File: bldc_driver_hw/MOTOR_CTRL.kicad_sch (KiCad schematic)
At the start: 18 parts, among them U3 DRV8328BRUYR

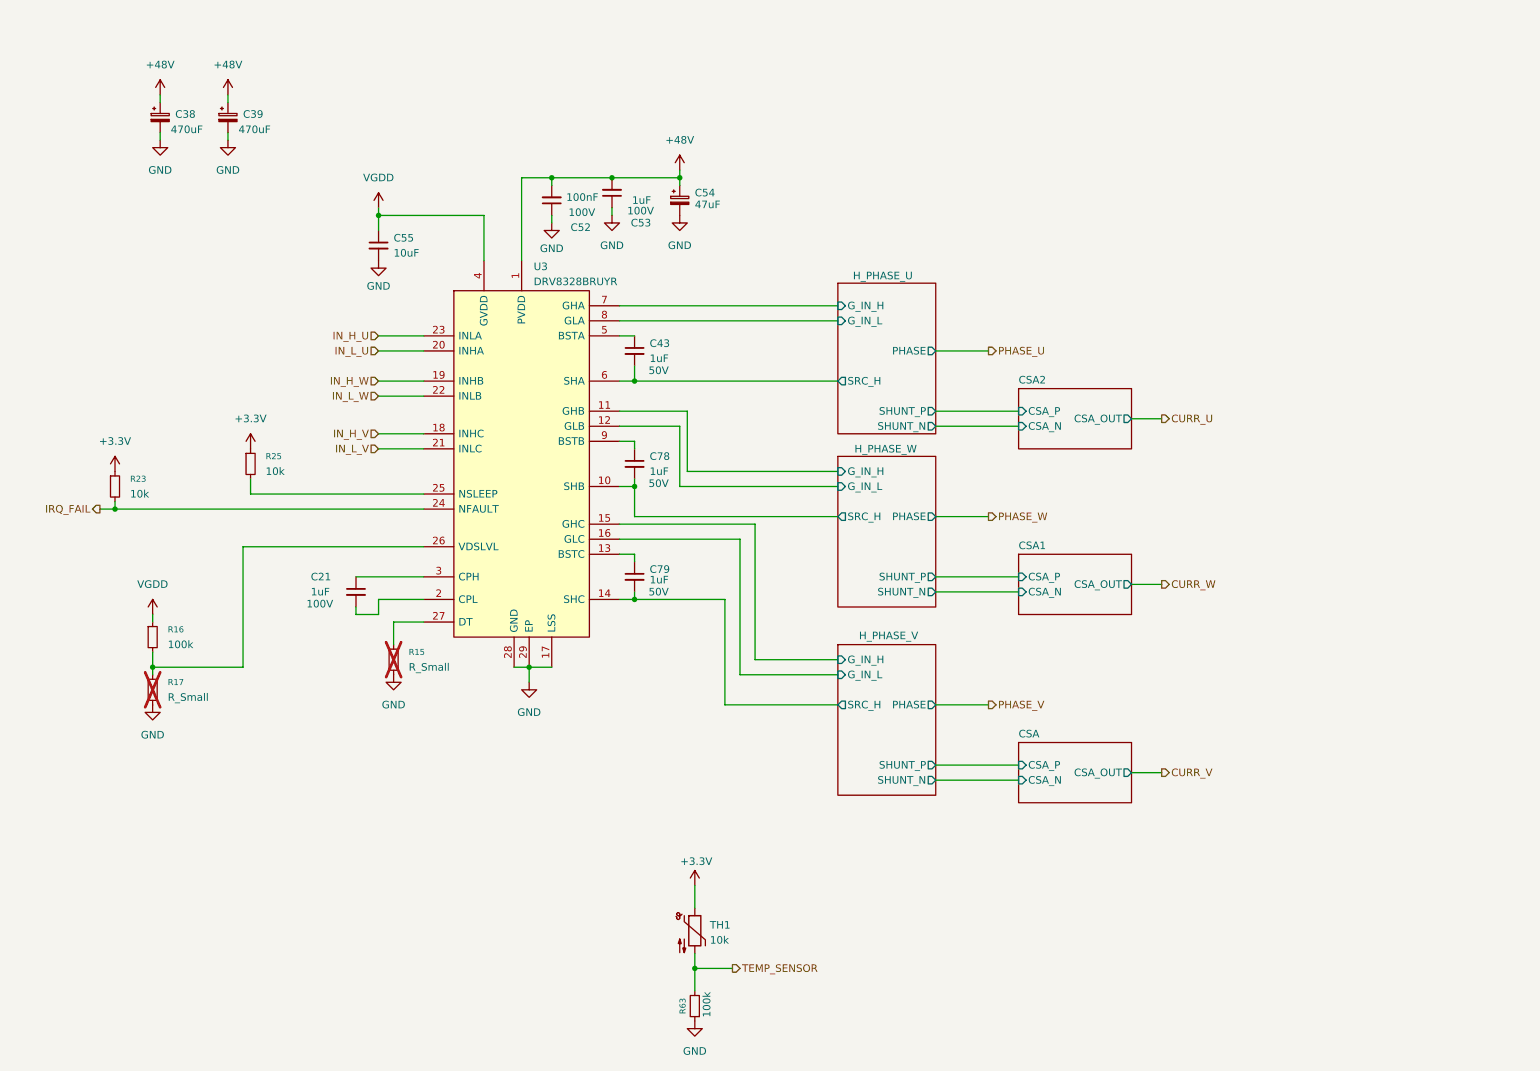
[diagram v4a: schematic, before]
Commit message: schematic finished pcb in progress
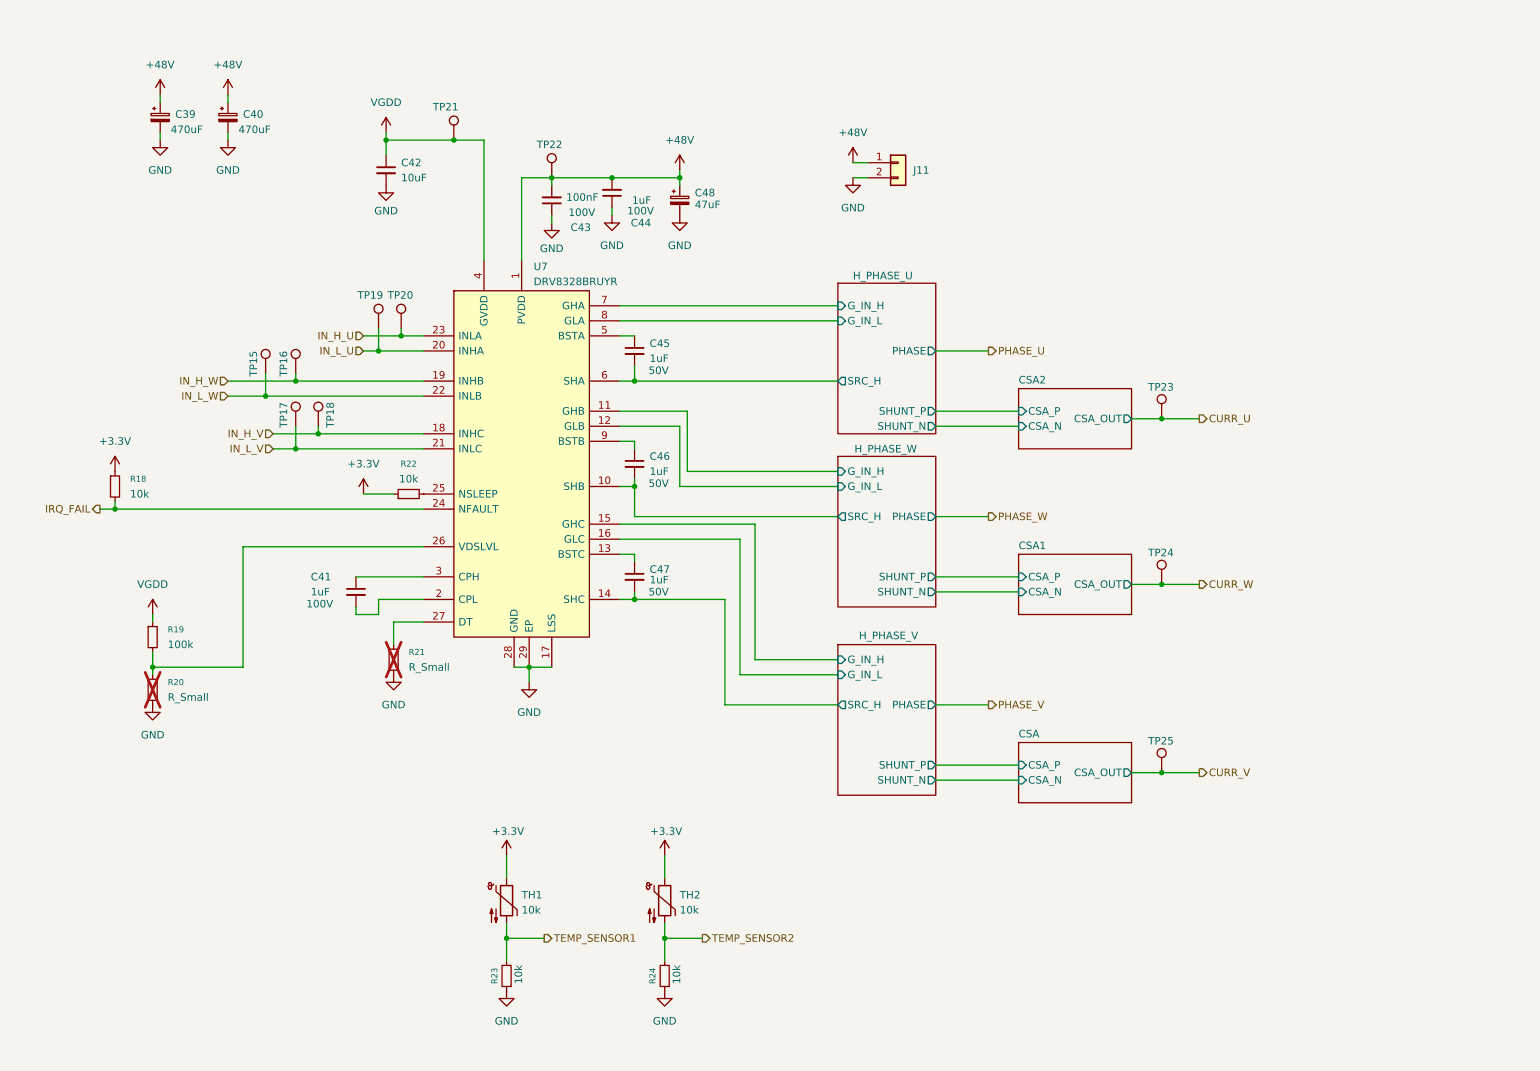
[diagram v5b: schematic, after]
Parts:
- added J11: Conn_01x02, Connector_AMASS:AMASS_XT60-F_1x02_P7.20mm_Vertical, symbol Connector_Generic:Conn_01x02
- added R24: 10k, Resistor_SMD:R_0805_2012Metric, symbol Device:R_Small
- added TH2: 10k, Resistor_SMD:R_0603_1608Metric, symbol Device:Thermistor_NTC
- added TP15, TP16, TP17, TP18, TP19, TP20, TP21, TP22, TP23, TP24, TP25: TestPoint, TestPoint:TestPoint_Pad_D2.0mm, symbol Connector:TestPoint
- C41: renamed from C21; footprint Capacitor_SMD:C_0805_2012Metric -> Capacitor_SMD:C_0603_1608Metric
- C45: renamed from C43; footprint Capacitor_SMD:C_0603_1608Metric_Pad1.08x0.95mm_HandSolder -> Capacitor_SMD:C_0603_1608Metric
- C46: renamed from C78; footprint Capacitor_SMD:C_0603_1608Metric_Pad1.08x0.95mm_HandSolder -> Capacitor_SMD:C_0603_1608Metric
- C47: renamed from C79; footprint Capacitor_SMD:C_0603_1608Metric_Pad1.08x0.95mm_HandSolder -> Capacitor_SMD:C_0603_1608Metric
- R23: renamed from R63; value 100k -> 10k
- renumbered C38 to C39, C39 to C40, C55 to C42, C52 to C43, C53 to C44, C54 to C48, R23 to R18, R16 to R19, R17 to R20, R15 to R21, R25 to R22, U3 to U7
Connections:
- net +3.3V: now also TH2.1
- net +48V: now also J11.1 (Pin_1), TP22.1
- net CURR_U: now also TP23.1
- net CURR_V: now also TP25.1
- net CURR_W: now also TP24.1
- net GND: now also J11.2 (Pin_2), R24.1
- net IN_H_U: now also TP20.1
- net IN_H_V: now also TP18.1
- net IN_H_W: now also TP16.1
- net IN_L_U: now also TP19.1
- net IN_L_V: now also TP17.1
- net IN_L_W: now also TP15.1
- net VGDD: now also TP21.1
- net TEMP_SENSOR renamed TEMP_SENSOR1
- new net TEMP_SENSOR2: R24.2, TH2.2
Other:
- moved on the sheet: C42, R22, R23, TH1
